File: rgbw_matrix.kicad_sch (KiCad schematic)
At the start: 36 parts, among them IC1 TLC59283DBQR, IC2 TLC59283DBQR, IC3 TLC59283DBQR, IC4 TLC59283DBQR, IC5 TLC59283DBQR, IC6 TLC59283DBQR

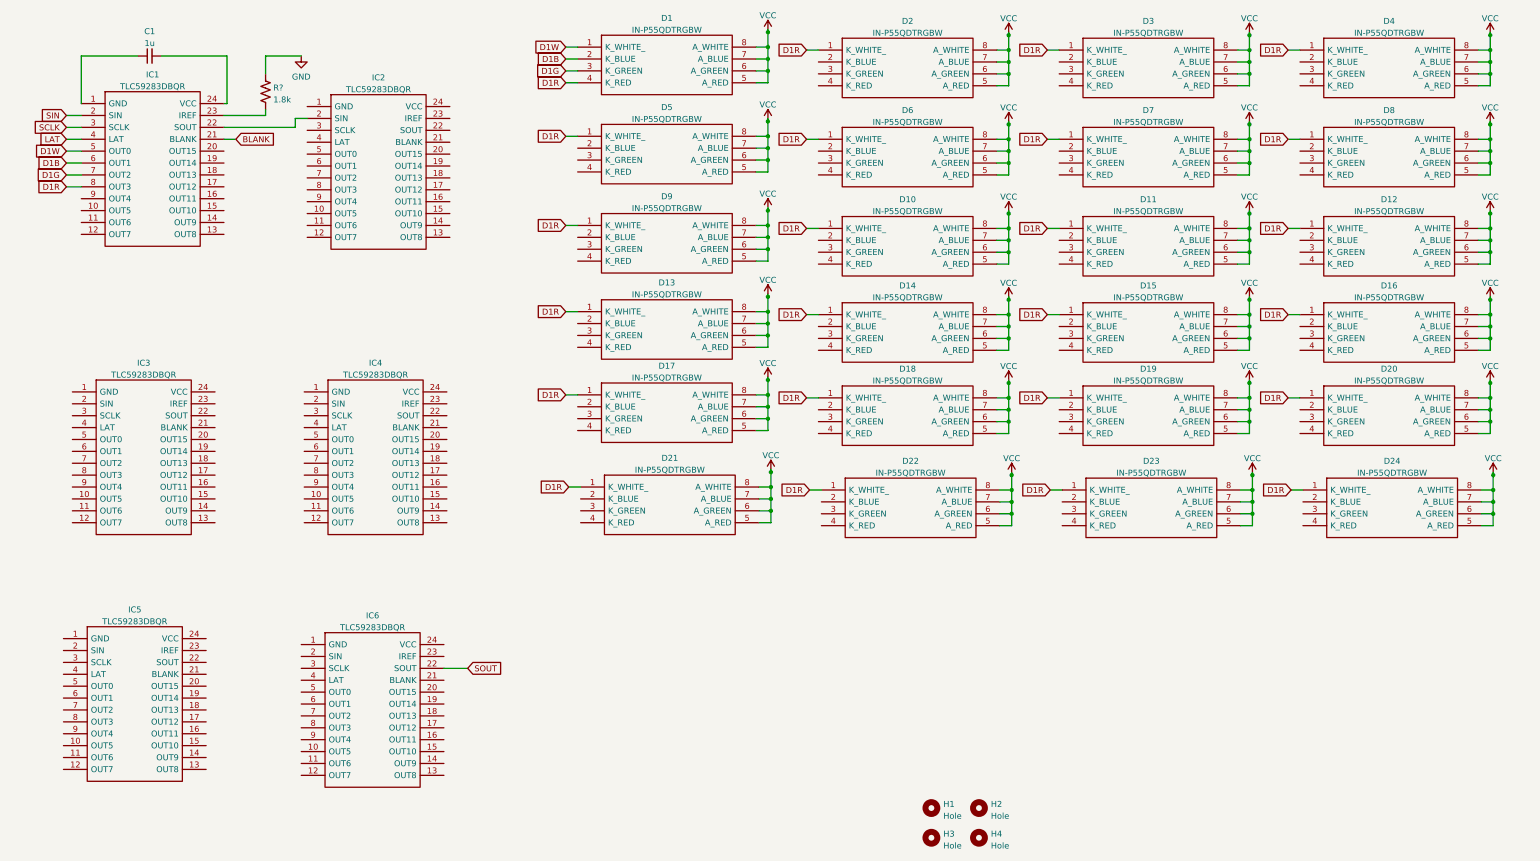
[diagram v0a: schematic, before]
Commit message: components connected v1
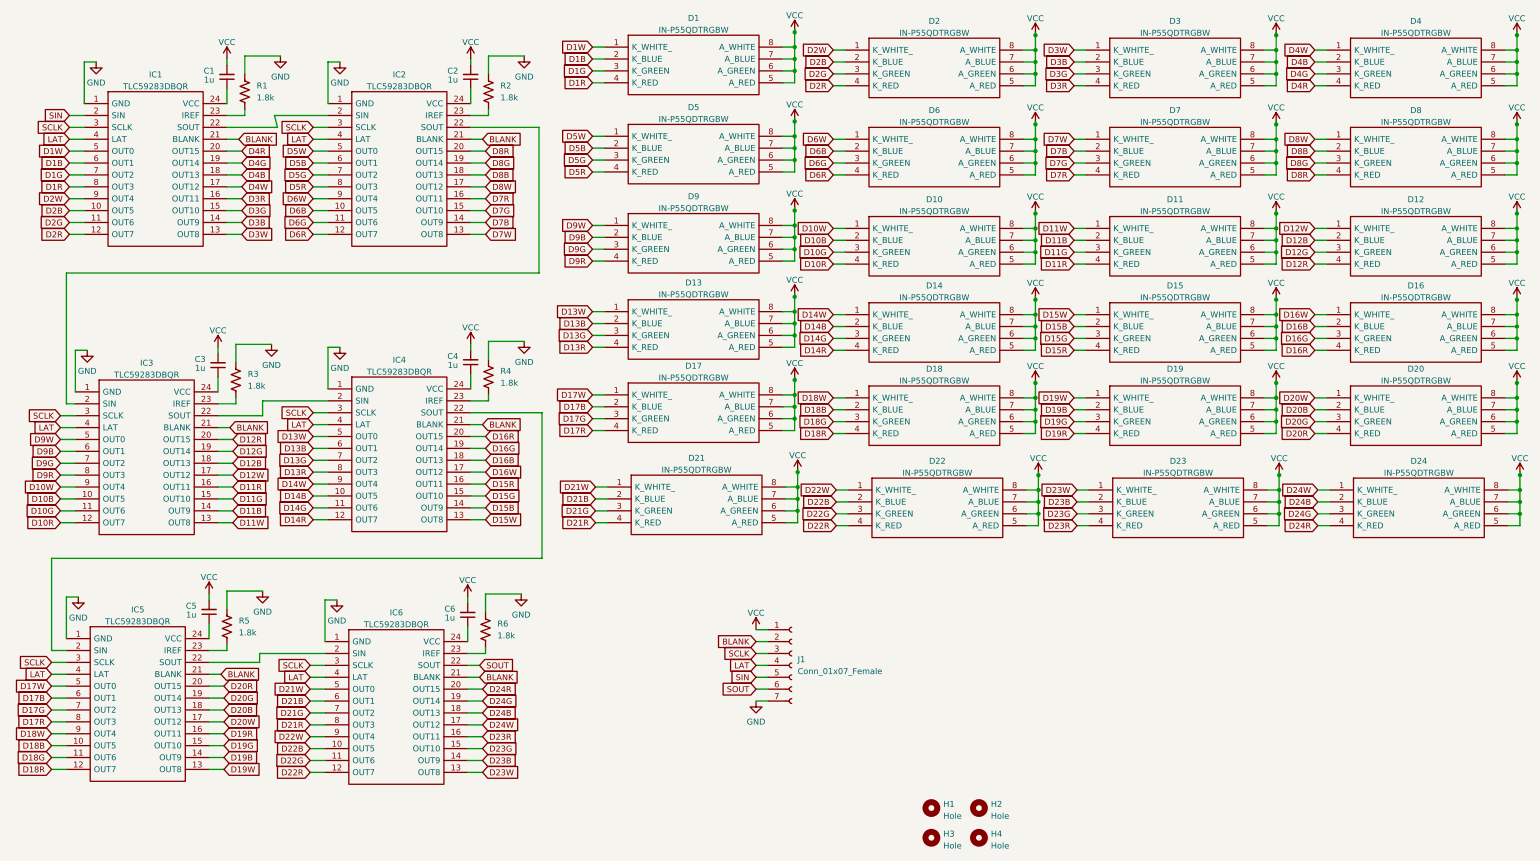
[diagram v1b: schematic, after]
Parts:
- removed R?: 1.8k, symbol Device:R_US
- added C2, C3, C4, C5, C6: 1u, Capacitor_SMD:C_0201_0603Metric, symbol Device:C_Small
- added J1: Conn_01x07_Female, Connector_PinHeader_2.54mm:PinHeader_1x07_P2.54mm_Vertical, symbol Connector:Conn_01x07_Female
- added R1, R2, R3, R4, R5, R6: 1.8k, Resistor_SMD:R_0201_0603Metric, symbol Device:1.8k
- C1: footprint (none) -> Capacitor_SMD:C_0201_0603Metric
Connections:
- net BLANK: now also IC2.21 (BLANK), IC3.21 (BLANK), IC4.21 (BLANK), IC5.21 (BLANK), IC6.21 (BLANK), J1.2 (Pin_2)
- net D1R: no longer D10.1 (K_WHITE_), D11.1 (K_WHITE_), D12.1 (K_WHITE_), D13.1 (K_WHITE_), D14.1 (K_WHITE_), D15.1 (K_WHITE_), D16.1 (K_WHITE_), D17.1 (K_WHITE_), D18.1 (K_WHITE_), D19.1 (K_WHITE_), D2.1 (K_WHITE_), D20.1 (K_WHITE_), D21.1 (K_WHITE_), D22.1 (K_WHITE_), D23.1 (K_WHITE_), D24.1 (K_WHITE_), D3.1 (K_WHITE_), D4.1 (K_WHITE_), D5.1 (K_WHITE_), D6.1 (K_WHITE_), D7.1 (K_WHITE_), D8.1 (K_WHITE_), D9.1 (K_WHITE_)
- net GND: now also IC1.1 (GND), IC2.1 (GND), IC3.1 (GND), IC4.1 (GND), IC5.1 (GND), IC6.1 (GND), J1.7 (Pin_7), R1.1, R2.1, R3.1, R4.1, R5.1, R6.1
- net LAT: now also IC2.4 (LAT), IC3.4 (LAT), IC4.4 (LAT), IC5.4 (LAT), IC6.4 (LAT), J1.4 (Pin_4)
- net SCLK: now also IC2.3 (SCLK), IC3.3 (SCLK), IC4.3 (SCLK), IC5.3 (SCLK), IC6.3 (SCLK), J1.3 (Pin_3)
- net SIN: now also J1.5 (Pin_5)
- net SOUT: now also J1.6 (Pin_6)
- net VCC: now also C1.2, C2.2, C3.2, C4.2, C5.2, C6.2, J1.1 (Pin_1)
- net D21B: now reaches D21.2 (K_BLUE)
- net D21B: now also IC6.6 (OUT1)
- net D21G: now reaches D21.3 (K_GREEN)
- net D21G: now also IC6.7 (OUT2)
- net D21R: now reaches D21.4 (K_RED)
- net D21R: now also IC6.8 (OUT3)
- net D22B: now reaches D22.2 (K_BLUE)
- net D22B: now also IC6.10 (OUT5)
- net D22G: now reaches D22.3 (K_GREEN)
- net D22G: now also IC6.11 (OUT6)
- net D22R: now reaches D22.4 (K_RED)
- net D22R: now also IC6.12 (OUT7)
- net D11B: now reaches D11.2 (K_BLUE)
- net D11B: now also IC3.14 (OUT9)
- net D11G: now reaches D11.3 (K_GREEN)
- net D11G: now also IC3.15 (OUT10)
- net D11R: now reaches D11.4 (K_RED)
- net D11R: now also IC3.16 (OUT11)
- net D10B: now reaches IC3.10 (OUT5)
- net D10B: now also D10.2 (K_BLUE)
- net D10G: now reaches IC3.11 (OUT6)
- net D10G: now also D10.3 (K_GREEN)
- net D10R: now reaches IC3.12 (OUT7)
- net D10R: now also D10.4 (K_RED)
- net D11W: now reaches IC3.13 (OUT8)
- net D11W: now also D11.1 (K_WHITE_)
- net D12W: now reaches IC3.17 (OUT12)
- net D12W: now also D12.1 (K_WHITE_)
- net D12B: now reaches IC3.18 (OUT13)
- net D12B: now also D12.2 (K_BLUE)
- net D12G: now reaches IC3.19 (OUT14)
- net D12G: now also D12.3 (K_GREEN)
- net at IC3.2 (SIN): now also IC2.22 (SOUT)
- net D12R: now reaches IC3.20 (OUT15)
- net D12R: now also D12.4 (K_RED)
- net at IC3.22 (SOUT): now also IC4.2 (SIN)
- net at IC3.23 (IREF): now also R3.2
- net at IC3.24 (VCC): now also C3.1
- net D9W: now reaches IC3.5 (OUT0)
- net D9W: now also D9.1 (K_WHITE_)
- net D9B: now reaches IC3.6 (OUT1)
- net D9B: now also D9.2 (K_BLUE)
- net D9G: now reaches IC3.7 (OUT2)
- net D9G: now also D9.3 (K_GREEN)
- net D9R: now reaches IC3.8 (OUT3)
- net D9R: now also D9.4 (K_RED)
- net D10W: now reaches IC3.9 (OUT4)
- net D10W: now also D10.1 (K_WHITE_)
- net D3B: now reaches D3.2 (K_BLUE)
- net D3B: now also IC1.14 (OUT9)
- net D3G: now reaches D3.3 (K_GREEN)
- net D3G: now also IC1.15 (OUT10)
- net D3R: now reaches D3.4 (K_RED)
- net D3R: now also IC1.16 (OUT11)
- net D6B: now reaches IC2.10 (OUT5)
- net D6B: now also D6.2 (K_BLUE)
- net D6G: now reaches IC2.11 (OUT6)
- net D6G: now also D6.3 (K_GREEN)
- net D6R: now reaches IC2.12 (OUT7)
- net D6R: now also D6.4 (K_RED)
- net D7W: now reaches IC2.13 (OUT8)
- net D7W: now also D7.1 (K_WHITE_)
- net D7B: now reaches IC2.14 (OUT9)
- net D7B: now also D7.2 (K_BLUE)
- net D7G: now reaches IC2.15 (OUT10)
- net D7G: now also D7.3 (K_GREEN)
- net D7R: now reaches IC2.16 (OUT11)
- net D7R: now also D7.4 (K_RED)
- net D8W: now reaches IC2.17 (OUT12)
- net D8W: now also D8.1 (K_WHITE_)
- net D8B: now reaches IC2.18 (OUT13)
- net D8B: now also D8.2 (K_BLUE)
- net D8G: now reaches IC2.19 (OUT14)
- net D8G: now also D8.3 (K_GREEN)
- net D8R: now reaches IC2.20 (OUT15)
- net D8R: now also D8.4 (K_RED)
- net at IC2.23 (IREF): now also R2.2
- net at IC2.24 (VCC): now also C2.1
- net D5W: now reaches IC2.5 (OUT0)
- net D5W: now also D5.1 (K_WHITE_)
- net D5B: now reaches IC2.6 (OUT1)
- net D5B: now also D5.2 (K_BLUE)
- net D5G: now reaches IC2.7 (OUT2)
- net D5G: now also D5.3 (K_GREEN)
- net D5R: now reaches IC2.8 (OUT3)
- net D5R: now also D5.4 (K_RED)
- net D6W: now reaches IC2.9 (OUT4)
- net D6W: now also D6.1 (K_WHITE_)
- net D16B: now reaches D16.2 (K_BLUE)
- net D16B: now also IC4.18 (OUT13)
- net D16G: now reaches D16.3 (K_GREEN)
- net D16G: now also IC4.19 (OUT14)
- net D16R: now reaches D16.4 (K_RED)
- net D16R: now also IC4.20 (OUT15)
- net D19B: now reaches D19.2 (K_BLUE)
- net D19B: now also IC5.14 (OUT9)
- net D19G: now reaches D19.3 (K_GREEN)
- net D19G: now also IC5.15 (OUT10)
- net D19R: now reaches D19.4 (K_RED)
- net D19R: now also IC5.16 (OUT11)
- net at C1.1: now also IC1.24 (VCC); no longer IC1.1 (GND)
- net D2B: now reaches IC1.10 (OUT5)
- net D2B: now also D2.2 (K_BLUE)
- net D2G: now reaches IC1.11 (OUT6)
- net D2G: now also D2.3 (K_GREEN)
- net D2R: now reaches IC1.12 (OUT7)
- net D2R: now also D2.4 (K_RED)
- net D3W: now reaches IC1.13 (OUT8)
- net D3W: now also D3.1 (K_WHITE_)
- net D4W: now reaches IC1.17 (OUT12)
- net D4W: now also D4.1 (K_WHITE_)
- net D4B: now reaches IC1.18 (OUT13)
- net D4B: now also D4.2 (K_BLUE)
- net D4G: now reaches IC1.19 (OUT14)
- net D4G: now also D4.3 (K_GREEN)
- net D4R: now reaches IC1.20 (OUT15)
- net D4R: now also D4.4 (K_RED)
- net at IC1.23 (IREF): now also R1.2
- net D2W: now reaches IC1.9 (OUT4)
- net D2W: now also D2.1 (K_WHITE_)
- net D14B: now reaches D14.2 (K_BLUE)
- net D14B: now also IC4.10 (OUT5)
- net D14G: now reaches D14.3 (K_GREEN)
- net D14G: now also IC4.11 (OUT6)
- net D14R: now reaches D14.4 (K_RED)
- net D14R: now also IC4.12 (OUT7)
- net D18B: now reaches IC5.10 (OUT5)
- net D18B: now also D18.2 (K_BLUE)
- net D18G: now reaches IC5.11 (OUT6)
- net D18G: now also D18.3 (K_GREEN)
- net D18R: now reaches IC5.12 (OUT7)
- net D18R: now also D18.4 (K_RED)
- net D19W: now reaches IC5.13 (OUT8)
- net D19W: now also D19.1 (K_WHITE_)
- net D20W: now reaches IC5.17 (OUT12)
- net D20W: now also D20.1 (K_WHITE_)
- net D20B: now reaches IC5.18 (OUT13)
- net D20B: now also D20.2 (K_BLUE)
- net D20G: now reaches IC5.19 (OUT14)
- net D20G: now also D20.3 (K_GREEN)
- net at IC5.2 (SIN): now also IC4.22 (SOUT)
- net D20R: now reaches IC5.20 (OUT15)
- net D20R: now also D20.4 (K_RED)
- net at IC5.22 (SOUT): now also IC6.2 (SIN)
- net at IC5.23 (IREF): now also R5.2
- net at IC5.24 (VCC): now also C5.1
- net D17W: now reaches IC5.5 (OUT0)
- net D17W: now also D17.1 (K_WHITE_)
- net D17B: now reaches IC5.6 (OUT1)
- net D17B: now also D17.2 (K_BLUE)
- net D17G: now reaches IC5.7 (OUT2)
- net D17G: now also D17.3 (K_GREEN)
- net D17R: now reaches IC5.8 (OUT3)
- net D17R: now also D17.4 (K_RED)
- net D18W: now reaches IC5.9 (OUT4)
- net D18W: now also D18.1 (K_WHITE_)
- net D15W: now reaches IC4.13 (OUT8)
- net D15W: now also D15.1 (K_WHITE_)
- net D15B: now reaches IC4.14 (OUT9)
- net D15B: now also D15.2 (K_BLUE)
- net D15G: now reaches IC4.15 (OUT10)
- net D15G: now also D15.3 (K_GREEN)
- net D15R: now reaches IC4.16 (OUT11)
- net D15R: now also D15.4 (K_RED)
- net D16W: now reaches IC4.17 (OUT12)
- net D16W: now also D16.1 (K_WHITE_)
- net at IC4.23 (IREF): now also R4.2
- net at IC4.24 (VCC): now also C4.1
- net D13W: now reaches IC4.5 (OUT0)
- net D13W: now also D13.1 (K_WHITE_)
- net D13B: now reaches IC4.6 (OUT1)
- net D13B: now also D13.2 (K_BLUE)
- net D13G: now reaches IC4.7 (OUT2)
- net D13G: now also D13.3 (K_GREEN)
- net D13R: now reaches IC4.8 (OUT3)
- net D13R: now also D13.4 (K_RED)
- net D14W: now reaches IC4.9 (OUT4)
- net D14W: now also D14.1 (K_WHITE_)
- net D23W: now reaches IC6.13 (OUT8)
- net D23W: now also D23.1 (K_WHITE_)
- net D23B: now reaches IC6.14 (OUT9)
- net D23B: now also D23.2 (K_BLUE)
- net D23G: now reaches IC6.15 (OUT10)
- net D23G: now also D23.3 (K_GREEN)
- net D23R: now reaches IC6.16 (OUT11)
- net D23R: now also D23.4 (K_RED)
- net D24W: now reaches IC6.17 (OUT12)
- net D24W: now also D24.1 (K_WHITE_)
- net D24B: now reaches IC6.18 (OUT13)
- net D24B: now also D24.2 (K_BLUE)
- net D24G: now reaches IC6.19 (OUT14)
- net D24G: now also D24.3 (K_GREEN)
- net D24R: now reaches IC6.20 (OUT15)
- net D24R: now also D24.4 (K_RED)
- net at IC6.23 (IREF): now also R6.2
- net at IC6.24 (VCC): now also C6.1
- net D21W: now reaches IC6.5 (OUT0)
- net D21W: now also D21.1 (K_WHITE_)
- net D22W: now reaches IC6.9 (OUT4)
- net D22W: now also D22.1 (K_WHITE_)
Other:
- moved on the sheet: C1, D1, D10, D11, D12, D13, D14, D15, D16, D17, D18, D19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
